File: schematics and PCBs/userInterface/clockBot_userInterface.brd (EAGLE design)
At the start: 67.3 x 32.7 mm, 6 parts, among them X1 5566-8

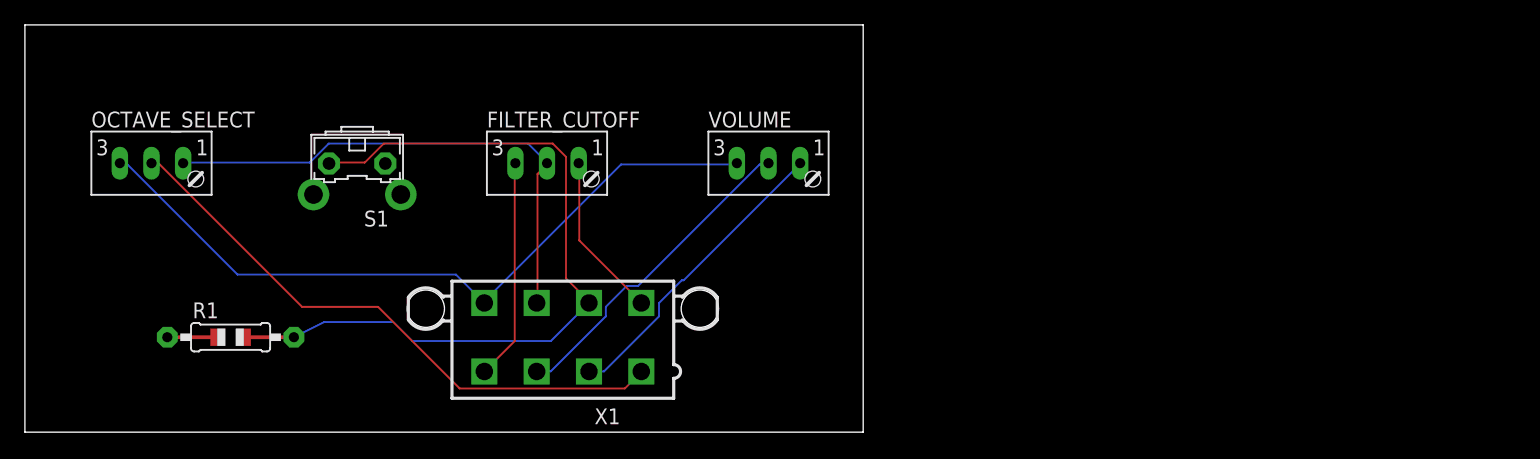
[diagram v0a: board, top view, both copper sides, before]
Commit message: User interface PCB update
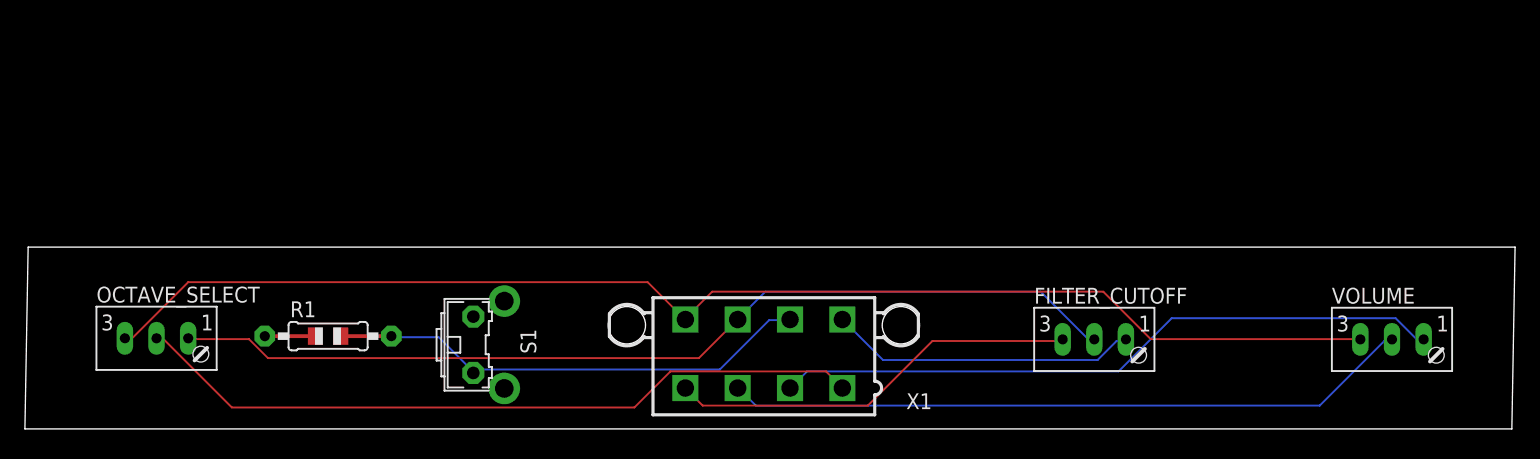
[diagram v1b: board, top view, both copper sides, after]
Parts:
- moved VOLUME 52.0 mm to (109.7, 6.18)
- moved FILTER_CUTOFF 46.2 mm to (85.8, 6.18)
- moved S1 17.0 mm to (37.2, 7.01), turned to 270 degrees
- moved X1 16.2 mm to (59.3, 6.29)
- moved OCTAVE_SELECT 14.1 mm to (10.6, 6.26)
- moved R1 7.83 mm to (24.3, 7.71)
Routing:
- net N$5: track 59.0 -> 104.8 mm
- net N$4: track 42.1 -> 77.2 mm
- net N$10: track 26.0 -> 55.4 mm
- net N$6: track 24.5 -> 53.9 mm
- net N$1: track 58.5 -> 35.1 mm
- net N$3: track 17.7 -> 33.1 mm
- net N$8: track 47.4 -> 59.1 mm
- net N$2: track 13.3 -> 24.8 mm
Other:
- board size 67.3 x 32.7 mm -> 119.6 x 14.6 mm
